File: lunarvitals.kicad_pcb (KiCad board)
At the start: 2 copper layers, 40 x 35 mm, 31 parts, among them J1 MLX90614, J2 SEN11574, J3 MAX30102, J4 ConductiveCord, U1 MPU-6050, U2 NRF52840-DONGLE, U3 AP2112K-3.3, U4 BMP280

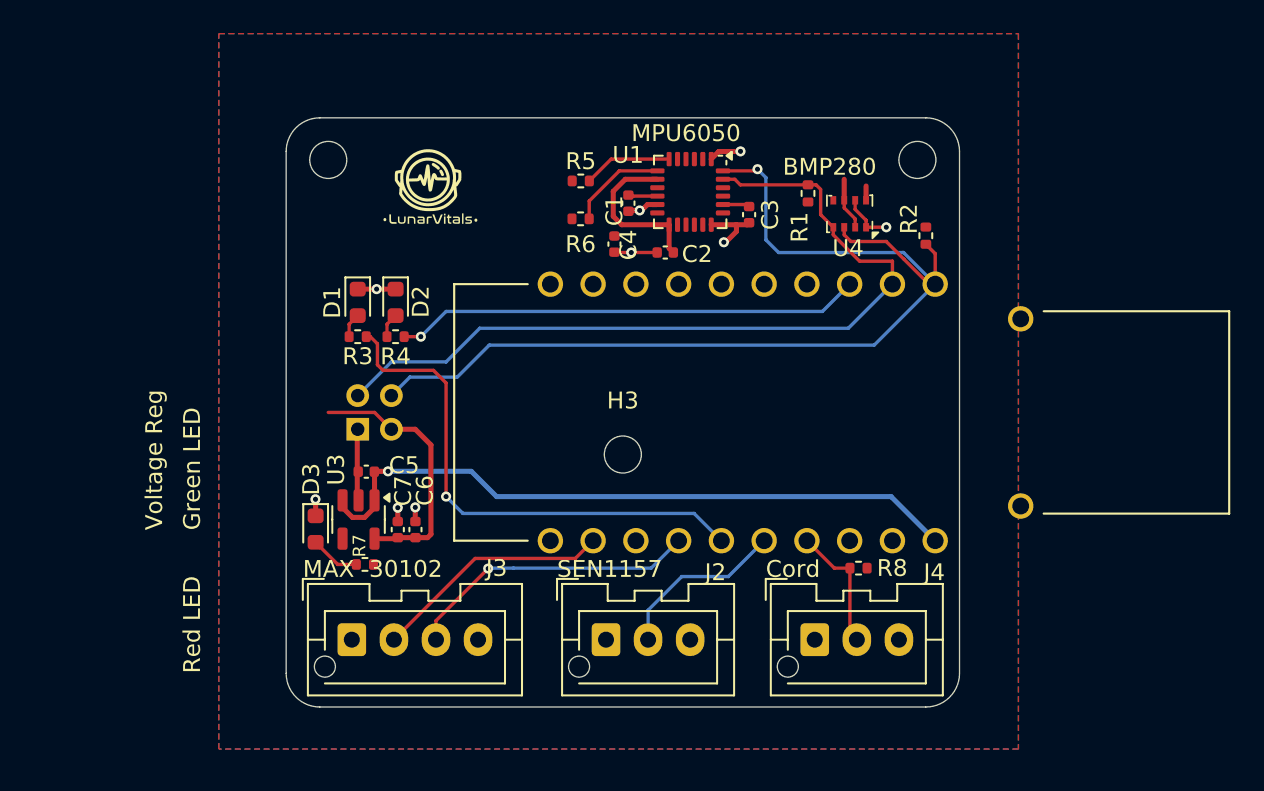
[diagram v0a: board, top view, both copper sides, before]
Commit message: PCB Updates
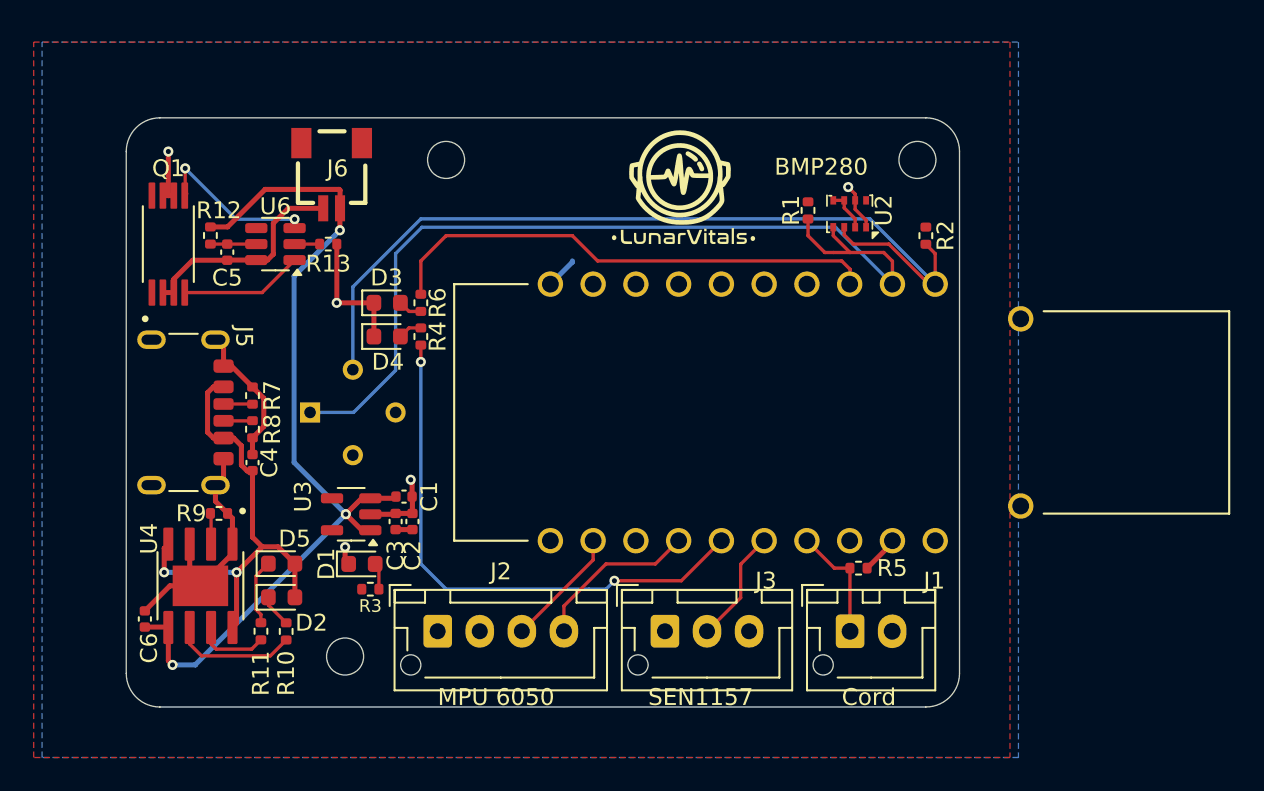
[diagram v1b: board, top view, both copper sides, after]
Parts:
- removed C7: 0.1uf, Capacitor_SMD:C_0402_1005Metric
- removed the G*** at (158.0, 96.5)
- removed J4: ConductiveCord, Connector_JST:JST_XA_B03B-XASK-1-A_1x03_P2.50mm_Vertical
- removed the R3 at (153.8, 105.5)
- removed the R5 at (167.0, 96.2)
- removed the U1 at (173.5, 96.9)
- added D2: Red_LED, LED_SMD:LED_0603_1608Metric, F.Cu at (149.2, 121.0)
- added D5: Blue_LED, LED_SMD:LED_0603_1608Metric, F.Cu at (149.2, 119.0)
- added G***: LOGO, lunar_vitals_custom:lunarvitals_logo_big, F.Cu at (173.0, 96.5)
- added J5: USB_C_Receptacle_PowerOnly_6P, Connector_USB:USB_C_Receptacle_GCT_USB4125-xx-x-0190_6P_TopMnt_Horizontal, F.Cu at (142.3, 110.0)
- added J6: Battery, SM02B-SRSS-TB_LF__SN_:SM02B-SRSS-TB_LF__SN_, F.Cu at (152.2, 95.9)
- added Q1: FS8205A, FS8205A:SOP65P640X120-8N, F.Cu at (142.5, 100.0)
- added R10: 1k, Resistor_SMD:R_0402_1005Metric, F.Cu at (149.5, 123.0)
- added R11: 1k, Resistor_SMD:R_0402_1005Metric, F.Cu at (148.0, 123.0)
- added R12: 100, Resistor_SMD:R_0402_1005Metric, F.Cu at (145.0, 99.5)
- added R13: 1k, Resistor_SMD:R_0402_1005Metric, F.Cu at (152.0, 100.0)
- added R7: 5.1k, Resistor_SMD:R_0402_1005Metric, F.Cu at (147.5, 109.0)
- added R8: 5.1k, Resistor_SMD:R_0402_1005Metric, F.Cu at (147.5, 111.0)
- added R9: 2.4k, Resistor_SMD:R_0402_1005Metric, F.Cu at (145.5, 116.0)
- added U4: TP4056, TP4056:SOP127P600X175-9N, F.Cu at (144.4, 120.3)
- added U5: MLX90614ESF-AAA-000-TU, MLX90614ESF-AAA-000-TU:TO254P912H435-4, B.Cu at (153.5, 110.0)
- added U6: DW01A, Package_TO_SOT_SMD:SOT-23-6, F.Cu at (148.9, 100.0)
- C1: value 10nf -> 4.7uf
- C2: value 0.1uf -> 10uf
- C3: value 2.2nf -> 0.1uf
- C5: value 4.7uf -> 0.1uf
- J1: value MLX90614 -> ConductiveCord; footprint Connector_PinSocket_2.00mm:PinSocket_2x02_P2.00mm_Vertical -> Connector_JST:JST_XH_B2B-XH-AM_1x02_P2.50mm_Vertical; moved to F.Cu
- J2: renamed from J3; value MAX30102 -> MPU6050; footprint Connector_JST:JST_XA_B04B-XASK-1-A_1x04_P2.50mm_Vertical -> Connector_JST:JST_XH_B4B-XH-AM_1x04_P2.50mm_Vertical
- J3: renamed from J2; footprint Connector_JST:JST_XA_B03B-XASK-1-A_1x03_P2.50mm_Vertical -> Connector_JST:JST_XH_B3B-XH-AM_1x03_P2.50mm_Vertical
- R6: value 4.7k -> 330
- moved J1 31.6 mm to (183.0, 123.0), turned to 0 degrees
- moved C3 27.8 mm to (156.0, 116.5), turned to 90 degrees
- moved C4 27.1 mm to (147.5, 113.0), turned to 90 degrees
- moved C2 21.9 mm to (157.0, 116.5), turned to 90 degrees
- moved H3 20.4 mm to (153.0, 124.5)
- moved C1 19.5 mm to (156.5, 115.0), turned to 0 degrees
- moved C6 16.9 mm to (141.1, 122.3)
- moved C5 15.4 mm to (146.0, 100.5), turned to -90 degrees
- moved R6 10.7 mm to (157.5, 103.5), turned to -90 degrees
- moved H1 7.00 mm to (159.0, 95.0)
- moved J2 5.12 mm to (158.5, 123.0)
- moved J3 3.54 mm to (172.0, 123.0)
- moved D1 3.44 mm to (154.0, 119.0), turned to 0 degrees
- moved D4 2.68 mm to (155.5, 105.5), turned to 0 degrees
- moved R3 1.50 mm to (154.5, 120.5), turned to 0 degrees
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- renumbered D3 to D1, D2 to D3, D1 to D4, R7 to R3, R8 to R5, U2 to U1, U4 to U2
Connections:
- C1 pad 1: +3.3V -> BOut+
- C3 pad 1: Net-(U1-CPOUT) -> +3.3V
- C4 pad 1: Net-(U1-REGOUT) -> +5V
- C5 pad 1: +5V -> Net-(U6-VCC)
- C5 pad 2: GND -> /B-
- C6 pad 1: +3.3V -> BOut+
- D3 pad 2: Net-(D2-A) -> Net-(D3-A)
- D4 pad 2: Net-(D1-A) (its old number) -> Net-(D4-A)
- J1 pad 1: GND -> /AIN7
- J1 pad 2: /I2C0_SCL -> +3.3V
- J2 pad 2: /I2C1_SDA -> GND
- J2 pad 3: /I2C1_SCL -> /I2C1_SDA
- J2 pad 4: GND -> /I2C1_SCL
- R4 pad 1: /GPIO17 -> /GPIO2
- R4 pad 2: Net-(D2-A) -> Net-(D4-A)
- R6 pad 1: +3.3V -> /GPIO17
- R6 pad 2: Net-(U1-AUX_CL) -> Net-(D3-A)
- U1 pad OUT: unconnected-(U2-PadOUT) -> +3.3V
- U1 pad VBUS: +5V -> unconnected-(U1-PadVBUS)
- U3 pad 1: +5V -> BOut+
- U3 pad 3: +5V -> BOut+
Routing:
- net BOut+: track 0.00 -> 53.3 mm, vias 0 -> 3
- net GND: track 22.2 -> 46.1 mm, vias 9 -> 5
- net +3.3V: track 29.7 -> 7.02 mm
- net /B-: track 0.00 -> 13.1 mm
- net +5V: track 40.1 -> 29.1 mm, vias 1 -> 2
- net Net-(U6-OC): track 0.00 -> 10.1 mm, vias 0 -> 2
- net /I2C0_SDA: track 62.4 -> 52.5 mm, vias 1 -> 0
- net /I2C1_SCL: track 17.5 -> 9.92 mm, vias 1 -> 0
- net Net-(U4-~{STDBY}): track 0.00 -> 7.39 mm
- net Net-(U6-OD): track 0.00 -> 7.32 mm
- net /I2C1_SDA: track 14.3 -> 7.13 mm
- net Net-(U1-AUX_CL): track 5.85 -> 0.00 mm
- net /I2C0_SCL: track 49.2 -> 54.7 mm
- net Net-(U1-AUX_DA): track 5.28 -> 0.00 mm
- net Net-(U4-~{CHRG}): track 0.00 -> 4.30 mm
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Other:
- board size 40 x 35 mm -> 49.5 x 35 mm
- board text added: "MPU 6050"
- board text removed: "Green LED"
- board text removed: "MAX 30102"
- board text removed: "MPU6050"
- board text removed: "Red LED"
- board text removed: "Voltage Reg"
